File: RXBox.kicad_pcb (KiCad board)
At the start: 4 copper layers, 56.6 x 17.8 mm, 75 parts, among them J1 SMA, J2 USB_A, U1 RTL2832U, U2 M24C02-WMN, U3 R820T2, U4 AP2112K-3.3, U5 74AUP1G74, U6 74LVC1G17, U7 USBLC6-2SC6, X1 19.2 MHz

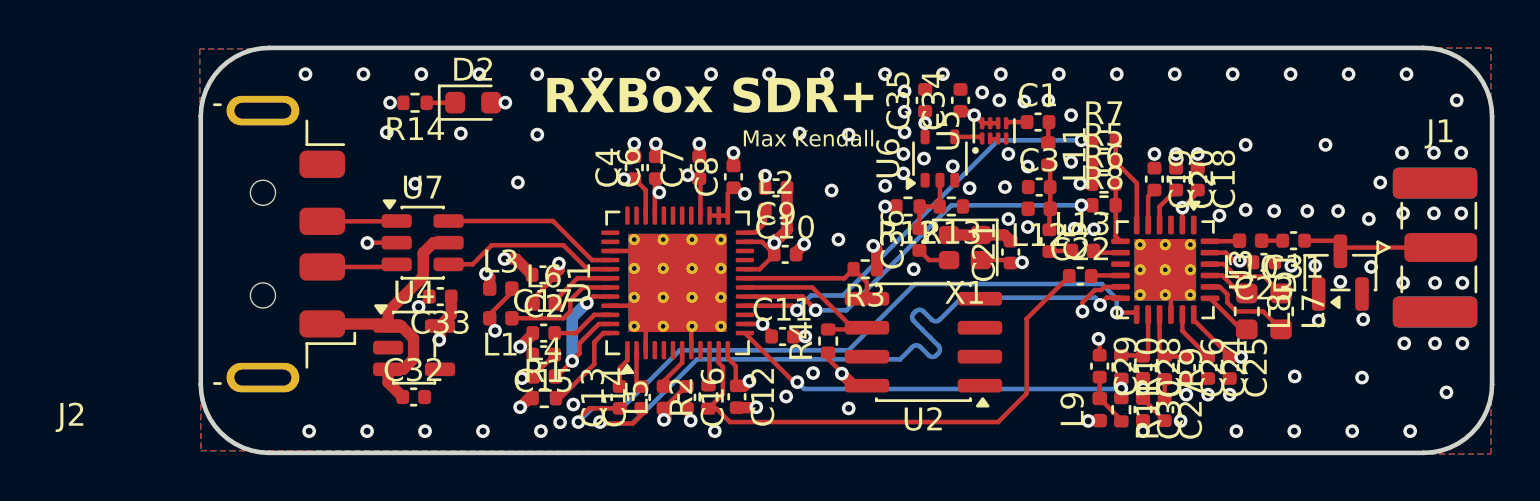
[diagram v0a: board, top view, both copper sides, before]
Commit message: lowkey forgot git exists
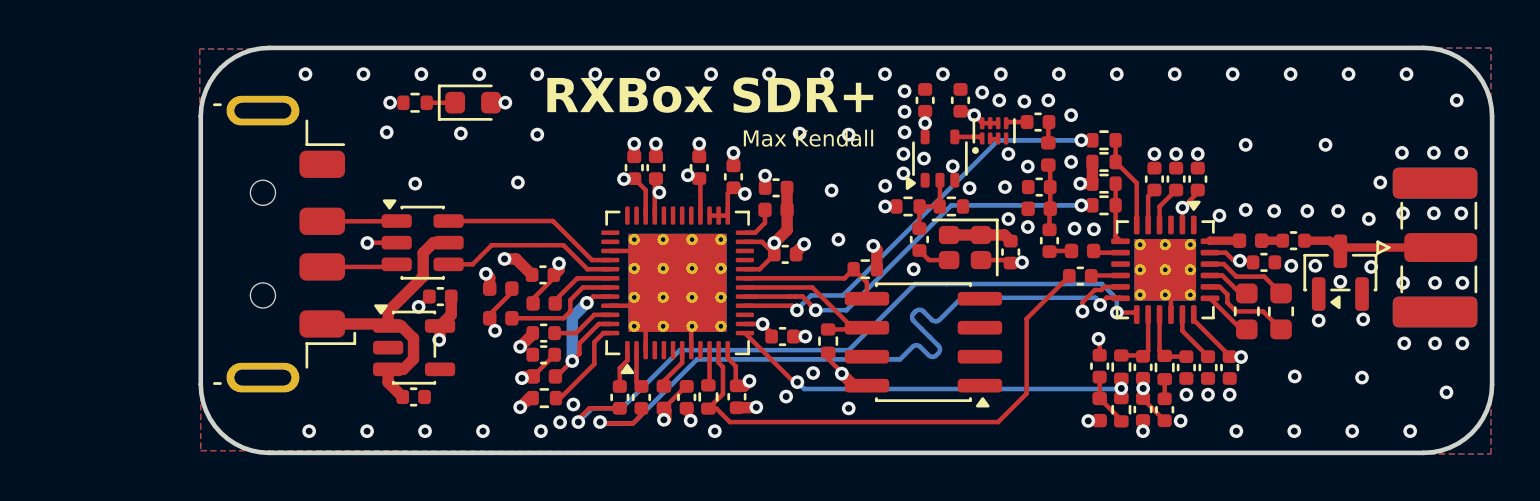
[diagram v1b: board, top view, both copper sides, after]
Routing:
- net Net-(U3-RF_IN): track 1.30 -> 2.60 mm
